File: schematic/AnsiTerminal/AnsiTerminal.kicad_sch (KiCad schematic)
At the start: 36 parts, among them J1 VGA_Output, J13 ManageDTR, J2 RS232

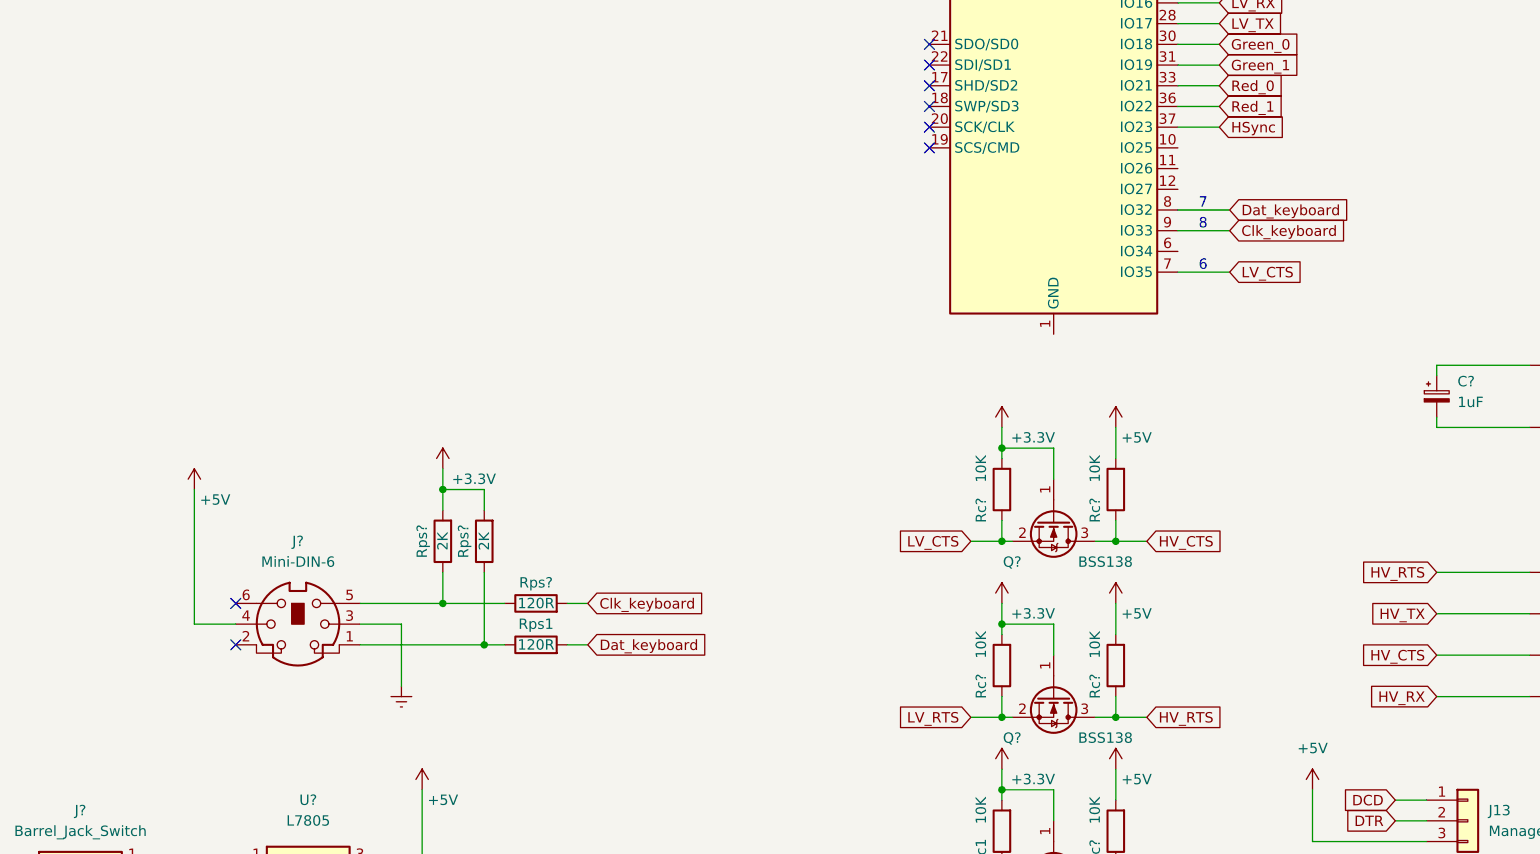
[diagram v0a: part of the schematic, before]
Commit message: Fix leds
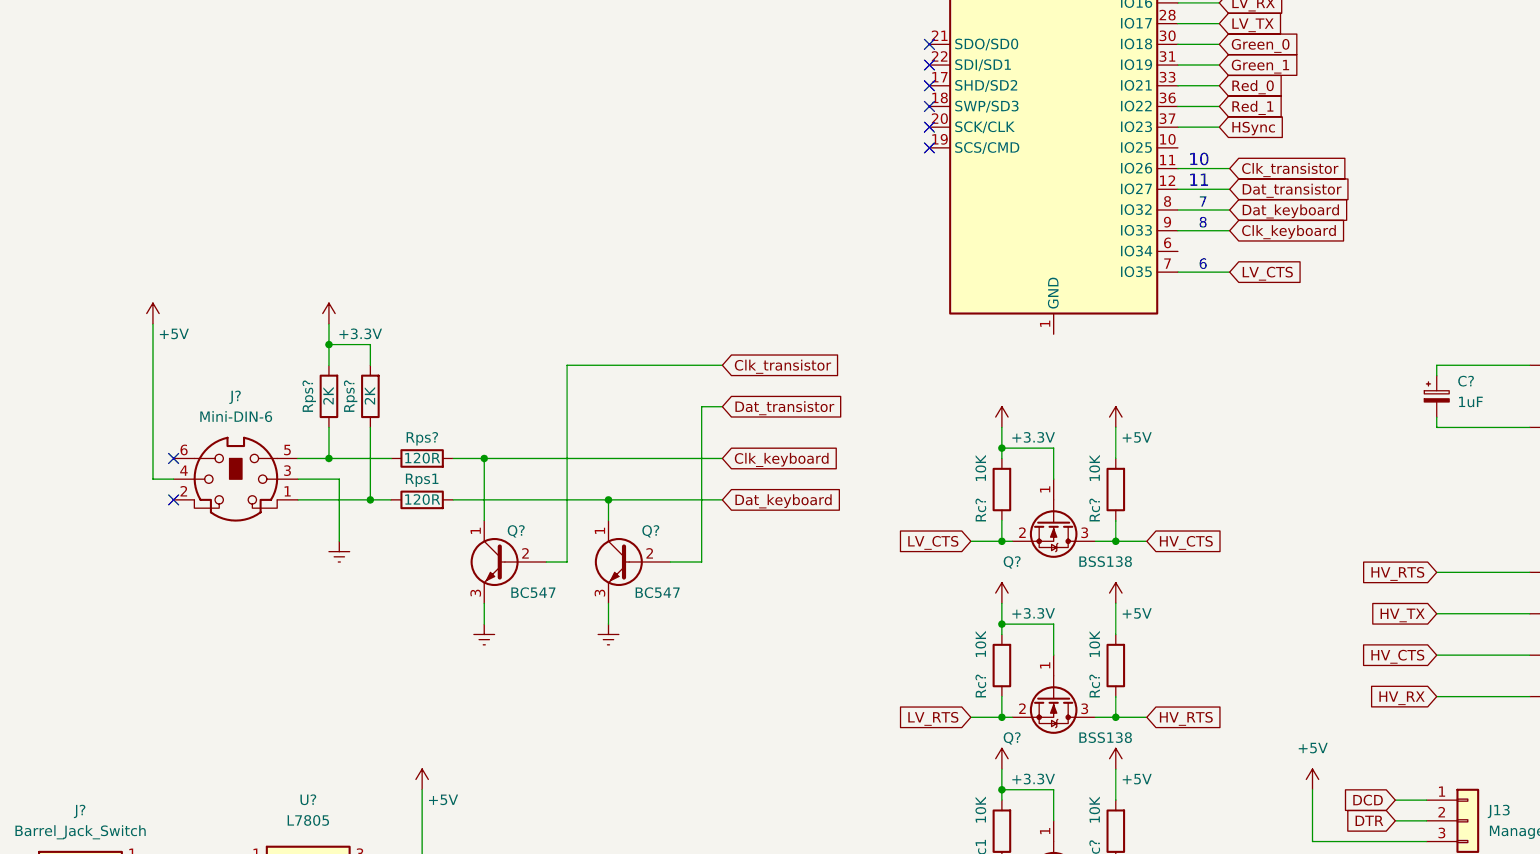
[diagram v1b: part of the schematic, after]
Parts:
- added Q? (x2): BC547, Package_TO_SOT_THT:TO-92_Inline, symbol Transistor_BJT:BC547
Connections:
- net Clk_keyboard: now also Q?.1 (C)
- net Dat_keyboard: now also Q?.1 (C)
- net GNDREF: now also Q?.3 (E), Q?.3 (E)
- net Clk_transistor: now reaches U?.11 (IO26)
- net Clk_transistor: now also Q?.2 (B)
- net Dat_transistor: now reaches U?.12 (IO27)
- net Dat_transistor: now also Q?.2 (B)
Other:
- note added: "10"
- note added: "11"
- moved on the sheet: J?, Rps1, Rps?
